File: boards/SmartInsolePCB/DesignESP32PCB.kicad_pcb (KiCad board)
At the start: 2 copper layers, 52 x 81.5 mm, 49 parts, among them J1 PJS008U-3000-0, J2 Conn_01x05_Socket, J3 Conn_02x10_Odd_Even, Q1 SS8050-G, Q2 SS8050-G, SW1 B3F-4000, SW2 B3F-4000, SW3 B3F-4000, SW4 B3F-4000, U1 D3V3XA4B10LP, U2 ESP32-S3-WROOM-1, U3 MPU-6050, U4 TLV75801PDRV

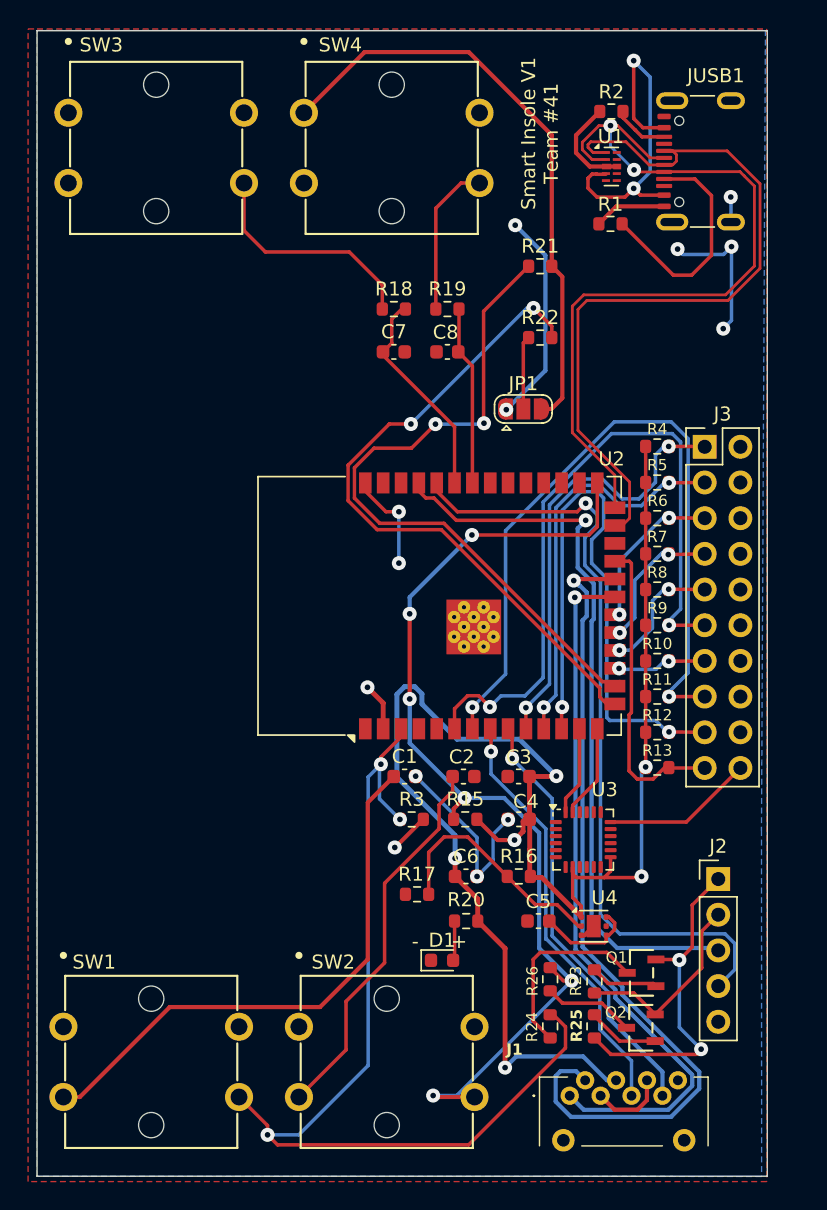
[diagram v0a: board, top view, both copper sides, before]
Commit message: changes
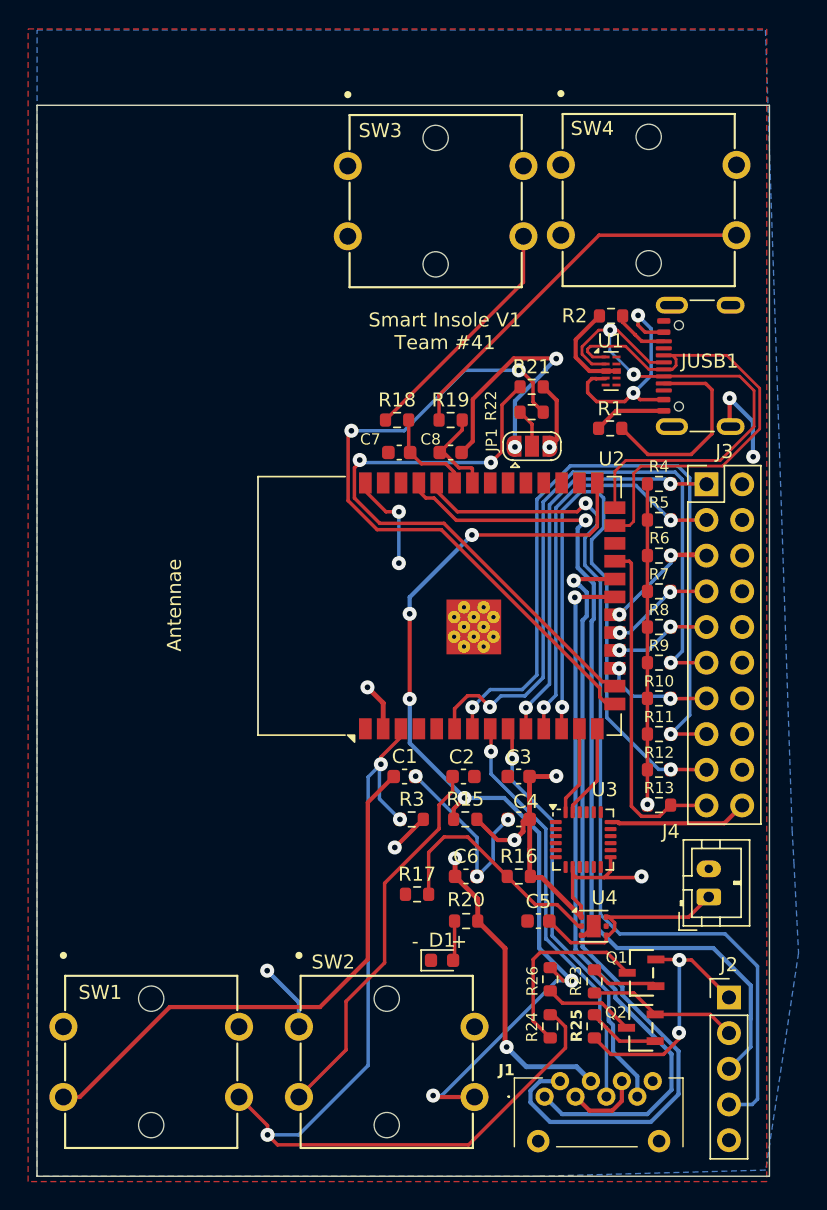
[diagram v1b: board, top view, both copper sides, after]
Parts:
- added J4: Conn_01x02_Pin, Connector_JST:JST_PH_B2B-PH-K_1x02_P2.00mm_Vertical, F.Cu at (139.0, 105.9)
- moved SW3 20.2 mm to (113.3, 53.8)
- moved SW4 18.7 mm to (128.5, 53.8)
- moved R1 14.6 mm to (132.0, 72.5)
- moved U1 14.6 mm to (132.0, 68.4)
- moved JUSB1 14.6 mm to (139.5, 68.1)
- moved R2 14.6 mm to (132.0, 64.5)
- moved R21 8.61 mm to (126.4, 69.5)
- moved J2 8.46 mm to (140.4, 113.0)
- moved R18 7.90 mm to (116.8, 71.9)
- moved R19 7.90 mm to (120.6, 71.9)
- moved C7 7.17 mm to (117.0, 74.2), turned to 180 degrees
- moved C8 7.17 mm to (120.6, 74.2), turned to 0 degrees
- moved R22 5.34 mm to (126.4, 71.3)
- moved JP1 2.72 mm to (126.4, 73.8)
- moved J3 2.67 mm to (138.8, 76.5)
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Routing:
- net /3V3: track 163.7 -> 86.6 mm, vias 8 -> 9
- net /USB_P: track 55.9 -> 36.1 mm
- net /USB_N: track 58.1 -> 39.0 mm
- net Net-(R19-Pad1): track 11.0 -> 27.7 mm
- net /RX: track 56.4 -> 66.8 mm
- net /TX: track 52.7 -> 62.5 mm
- net /End Hike: track 15.3 -> 6.85 mm
- net /POWER FROM BATTERY: track 7.16 -> 15.1 mm
- net /5VUSB: track 24.9 -> 17.4 mm
- net /GPIO46_STRAPPING: track 49.4 -> 42.6 mm
- net /Start Hike: track 12.8 -> 6.78 mm
- net /RTS: track 24.6 -> 18.9 mm
- net /DTR: track 13.9 -> 10.8 mm
- net /GPIO1: track 31.9 -> 29.0 mm
- net Net-(JP1-C): track 5.24 -> 2.78 mm
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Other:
- board size 52 x 81.5 mm -> 52.1 x 76.2 mm
- board text added: "Antennae"
